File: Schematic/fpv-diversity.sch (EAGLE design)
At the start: 62 parts, among them U1 LM1881M/NOPB, U2 LM1881M/NOPB, U3 LM1881M/NOPB, U4 MAX4545CAP+, U5 LT6206CMS8PBF, U6 LM1117IMP-5.0-NOPB

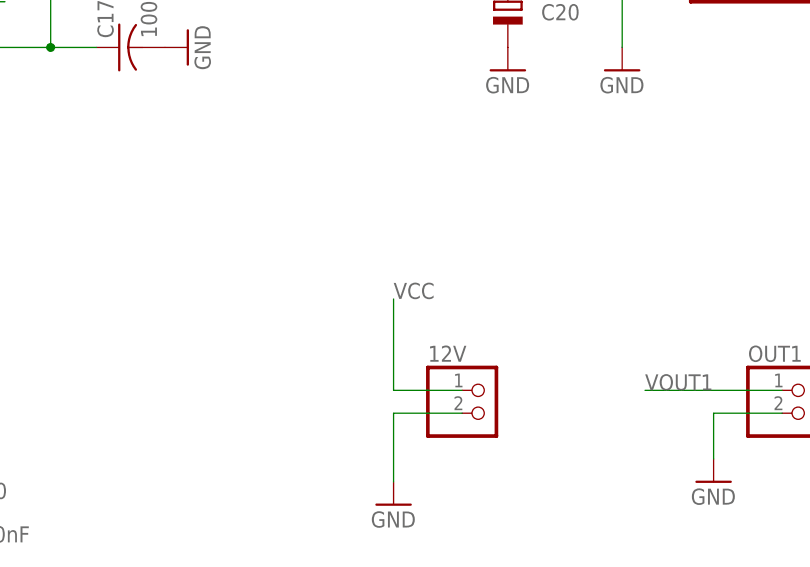
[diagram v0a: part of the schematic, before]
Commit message: Updates
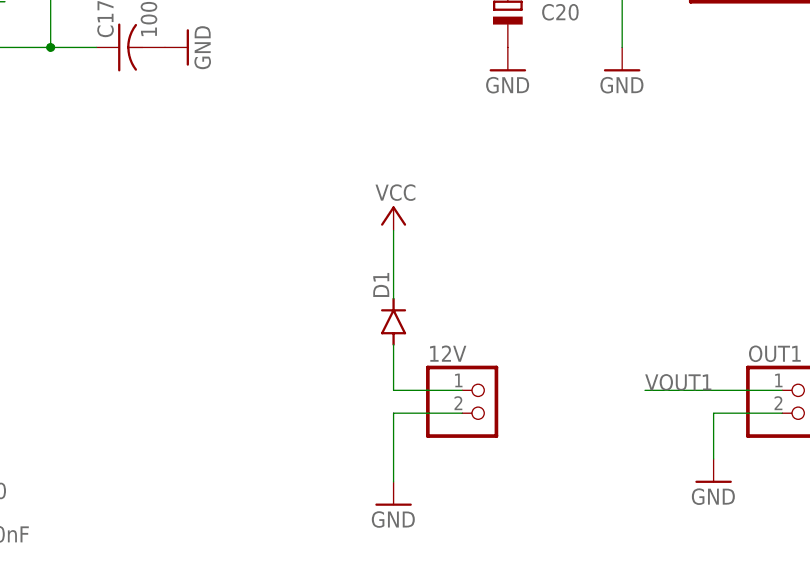
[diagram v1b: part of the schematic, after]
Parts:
- added D1: (no value), diode:DIODE-DO-214AC
- C19, C20: device rcl:CPOL-EUUD-4X5,8 -> rcl:CPOL-EUD/7343-31W
- R1, R10, R11, R12, R14, R15, R17, R18, R3, R7, R8: device rcl:R-US_R1206 -> rcl:R-US_R0805
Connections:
- new net N$6: 12V.1, D1.A
- net VCC: now also D1.C; no longer 12V.1

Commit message: more updates
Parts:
- R13, R2, R9: device rcl:R-US_R1206 -> rcl:R-US_R0805
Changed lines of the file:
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@@
 <part name="C3" library="rcl" library_urn="urn:adsk.eagle:library:334" deviceset="C-US" device="C0805" package3d_urn="urn:adsk.eagle:package:23617/2" value="100nF"/>
 <part name="GND3" library="supply1" library_urn="urn:adsk.eagle:library:371" deviceset="GND" device=""/>
-<part name="R2" library="rcl" library_urn="urn:adsk.eagle:library:334" deviceset="R-US_" device="R1206" package3d_urn="urn:adsk.eagle:package:23540/2" value="75"/>
+<part name="R2" library="rcl" library_urn="urn:adsk.eagle:library:334" deviceset="R-US_" device="R0805" package3d_urn="urn:adsk.eagle:package:23553/2" value="75"/>
 <part name="GND4" library="supply1" library_urn="urn:adsk.eagle:library:371" deviceset="GND" device=""/>
 <part name="U2" library="LM1881M_NOPB" deviceset="LM1881M/NOPB" device="" package3d_urn="urn:adsk.eagle:package:18494142/1"/>
@@
 <part name="C7" library="rcl" library_urn="urn:adsk.eagle:library:334" deviceset="C-US" device="C0805" package3d_urn="urn:adsk.eagle:package:23617/2" value="100nF"/>
 <part name="GND8" library="supply1" library_urn="urn:adsk.eagle:library:371" deviceset="GND" device=""/>
-<part name="R9" library="rcl" library_urn="urn:adsk.eagle:library:334" deviceset="R-US_" device="R1206" package3d_urn="urn:adsk.eagle:package:23540/2" value="75"/>
+<part name="R9" library="rcl" library_urn="urn:adsk.eagle:library:334" deviceset="R-US_" device="R0805" package3d_urn="urn:adsk.eagle:package:23553/2" value="75"/>
 <part name="GND9" library="supply1" library_urn="urn:adsk.eagle:library:371" deviceset="GND" device=""/>
 <part name="U3" library="LM1881M_NOPB" deviceset="LM1881M/NOPB" device="" package3d_urn="urn:adsk.eagle:package:18494142/1"/>
@@
 <part name="C13" library="rcl" library_urn="urn:adsk.eagle:library:334" deviceset="C-US" device="C0805" package3d_urn="urn:adsk.eagle:package:23617/2" value="100nF"/>
 <part name="GND20" library="supply1" library_urn="urn:adsk.eagle:library:371" deviceset="GND" device=""/>
-<part name="R13" library="rcl" library_urn="urn:adsk.eagle:library:334" deviceset="R-US_" device="R1206" package3d_urn="urn:adsk.eagle:package:23540/2" value="75"/>
+<part name="R13" library="rcl" library_urn="urn:adsk.eagle:library:334" deviceset="R-US_" device="R0805" package3d_urn="urn:adsk.eagle:package:23553/2" value="75"/>
 <part name="GND21" library="supply1" library_urn="urn:adsk.eagle:library:371" deviceset="GND" device=""/>
 <part name="U1" library="LM1881M_NOPB" deviceset="LM1881M/NOPB" device="" package3d_urn="urn:adsk.eagle:package:18494142/1"/>

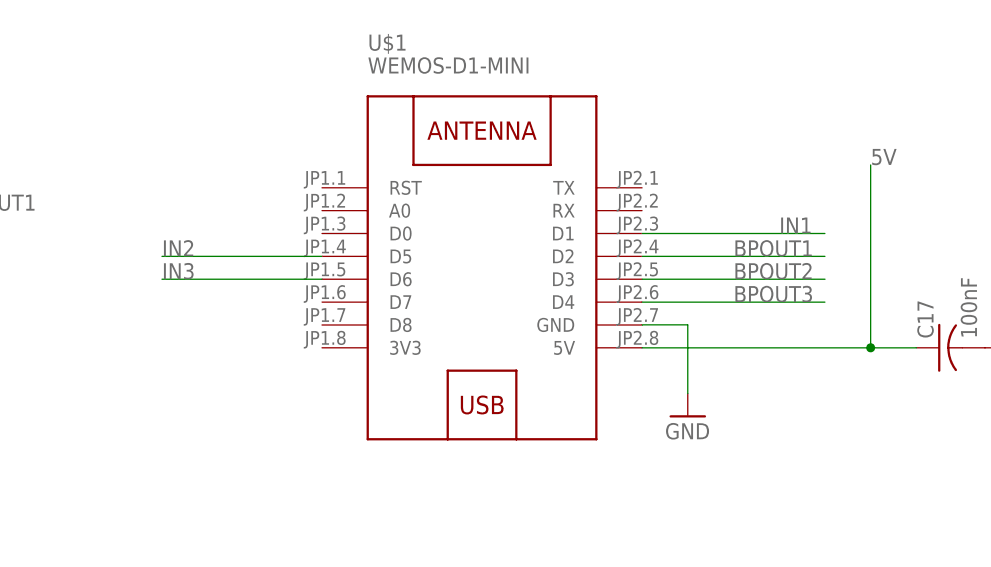
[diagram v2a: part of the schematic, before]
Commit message: Latest
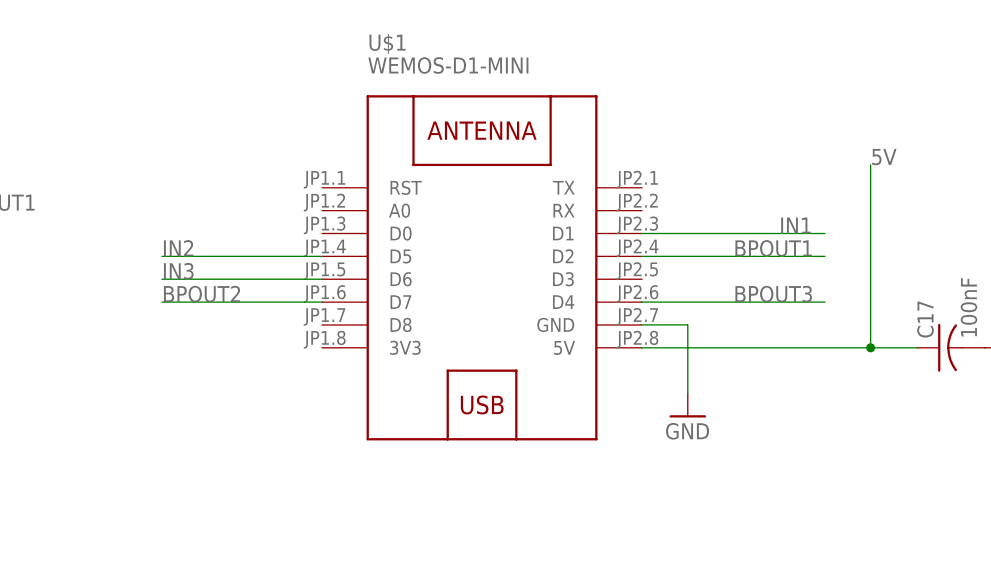
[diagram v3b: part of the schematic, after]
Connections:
- net BPOUT2: now also U$1.D7; no longer U$1.D3
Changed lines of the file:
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@@
 <grid distance="0.1" unitdist="inch" unit="inch" style="lines" multiple="1" display="no" altdistance="0.01" altunitdist="inch" altunit="inch"/>
 <layers>
-<layer number="1" name="Top" color="4" fill="1" visible="yes" active="no"/>
-<layer number="2" name="Route2" color="16" fill="1" visible="yes" active="no"/>
-<layer number="3" name="Route3" color="17" fill="1" visible="yes" active="no"/>
-<layer number="4" name="Route4" color="18" fill="1" visible="yes" active="no"/>
-<layer number="5" name="Route5" color="19" fill="1" visible="yes" active="no"/>
-<layer number="6" name="Route6" color="25" fill="1" visible="yes" active="no"/>
-<layer number="7" name="Route7" color="26" fill="1" visible="yes" active="no"/>
-<layer number="8" name="Route8" color="27" fill="1" visible="yes" active="no"/>
-<layer number="9" name="Route9" color="28" fill="1" visible="yes" active="no"/>
-<layer number="10" name="Route10" color="29" fill="1" visible="yes" active="no"/>
-<layer number="11" name="Route11" color="30" fill="1" visible="yes" active="no"/>
-<layer number="12" name="Route12" color="20" fill="1" visible="yes" active="no"/>
-<layer number="13" name="Route13" color="21" fill="1" visible="yes" active="no"/>
-<layer number="14" name="Route14" color="22" fill="1" visible="yes" active="no"/>
-<layer number="15" name="Route15" color="23" fill="1" visible="yes" active="no"/>
-<layer number="16" name="Bottom" color="1" fill="1" visible="yes" active="no"/>
-<layer number="17" name="Pads" color="2" fill="1" visible="yes" active="no"/>
-<layer number="18" name="Vias" color="2" fill="1" visible="yes" active="no"/>
-<layer number="19" name="Unrouted" color="6" fill="1" visible="yes" active="no"/>
-<layer number="20" name="Dimension" color="24" fill="1" visible="yes" active="no"/>
-<layer number="21" name="tPlace" color="7" fill="1" visible="yes" active="no"/>
-<layer number="22" name="bPlace" color="7" fill="1" visible="yes" active="no"/>
-<layer number="23" name="tOrigins" color="15" fill="1" visible="yes" active="no"/>
-<layer number="24" name="bOrigins" color="15" fill="1" visible="yes" active="no"/>
-<layer number="25" name="tNames" color="7" fill="1" visible="yes" active="no"/>
-<layer number="26" name="bNames" color="7" fill="1" visible="yes" active="no"/>
-<layer number="27" name="tValues" color="7" fill="1" visible="yes" active="no"/>
-<layer number="28" name="bValues" color="7" fill="1" visible="yes" active="no"/>
+<layer number="1" name="Top" color="4" fill="1" visible="no" active="no"/>
+<layer number="2" name="Route2" color="16" fill="1" visible="no" active="no"/>
+<layer number="3" name="Route3" color="17" fill="1" visible="no" active="no"/>
+<layer number="4" name="Route4" color="18" fill="1" visible="no" active="no"/>
+<layer number="5" name="Route5" color="19" fill="1" visible="no" active="no"/>
+<layer number="6" name="Route6" color="25" fill="1" visible="no" active="no"/>
+<layer number="7" name="Route7" color="26" fill="1" visible="no" active="no"/>
+<layer number="8" name="Route8" color="27" fill="1" visible="no" active="no"/>
+<layer number="9" name="Route9" color="28" fill="1" visible="no" active="no"/>
+<layer number="10" name="Route10" color="29" fill="1" visible="no" active="no"/>
+<layer number="11" name="Route11" color="30" fill="1" visible="no" active="no"/>
+<layer number="12" name="Route12" color="20" fill="1" visible="no" active="no"/>
+<layer number="13" name="Route13" color="21" fill="1" visible="no" active="no"/>
+<layer number="14" name="Route14" color="22" fill="1" visible="no" active="no"/>
+<layer number="15" name="Route15" color="23" fill="1" visible="no" active="no"/>
+<layer number="16" name="Bottom" color="1" fill="1" visible="no" active="no"/>
+<layer number="17" name="Pads" color="2" fill="1" visible="no" active="no"/>
+<layer number="18" name="Vias" color="2" fill="1" visible="no" active="no"/>
+<layer number="19" name="Unrouted" color="6" fill="1" visible="no" active="no"/>
+<layer number="20" name="Dimension" color="24" fill="1" visible="no" active="no"/>
+<layer number="21" name="tPlace" color="7" fill="1" visible="no" active="no"/>
+<layer number="22" name="bPlace" color="7" fill="1" visible="no" active="no"/>
+<layer number="23" name="tOrigins" color="15" fill="1" visible="no" active="no"/>
+<layer number="24" name="bOrigins" color="15" fill="1" visible="no" active="no"/>
+<layer number="25" name="tNames" color="7" fill="1" visible="no" active="no"/>
+<layer number="26" name="bNames" color="7" fill="1" visible="no" active="no"/>
+<layer number="27" name="tValues" color="7" fill="1" visible="no" active="no"/>
+<layer number="28" name="bValues" color="7" fill="1" visible="no" active="no"/>
 <layer number="29" name="tStop" color="7" fill="3" visible="no" active="no"/>
 <layer number="30" name="bStop" color="7" fill="6" visible="no" active="no"/>
@@
 <layer number="35" name="tGlue" color="7" fill="4" visible="no" active="no"/>
 <layer number="36" name="bGlue" color="7" fill="5" visible="no" active="no"/>
-<layer number="37" name="tTest" color="7" fill="1" visible="yes" active="no"/>
-<layer number="38" name="bTest" color="7" fill="1" visible="yes" active="no"/>
+<layer number="37" name="tTest" color="7" fill="1" visible="no" active="no"/>
+<layer number="38" name="bTest" color="7" fill="1" visible="no" active="no"/>
 <layer number="39" name="tKeepout" color="4" fill="11" visible="no" active="no"/>
 <layer number="40" name="bKeepout" color="1" fill="11" visible="no" active="no"/>
@@
 <layer number="44" name="Drills" color="7" fill="1" visible="no" active="no"/>
 <layer number="45" name="Holes" color="7" fill="1" visible="no" active="no"/>
-<layer number="46" name="Milling" color="3" fill="1" visible="yes" active="no"/>
-<layer number="47" name="Measures" color="7" fill="1" visible="yes" active="no"/>
-<layer number="48" name="Document" color="7" fill="1" visible="yes" active="no"/>
-<layer number="49" name="Reference" color="7" fill="1" visible="yes" active="no"/>
-<layer number="51" name="tDocu" color="7" fill="1" visible="yes" active="no"/>
-<layer number="52" name="bDocu" color="7" fill="1" visible="yes" active="no"/>
+<layer number="46" name="Milling" color="3" fill="1" visible="no" active="no"/>
+<layer number="47" name="Measures" color="7" fill="1" visible="no" active="no"/>
+<layer number="48" name="Document" color="7" fill="1" visible="no" active="no"/>
+<layer number="49" name="Reference" color="7" fill="1" visible="no" active="no"/>
+<layer number="51" name="tDocu" color="7" fill="1" visible="no" active="no"/>
+<layer number="52" name="bDocu" color="7" fill="1" visible="no" active="no"/>
 <layer number="88" name="SimResults" color="9" fill="1" visible="yes" active="yes"/>
 <layer number="89" name="SimProbes" color="9" fill="1" visible="yes" active="yes"/>
@@
 <part name="GND11" library="supply1" library_urn="urn:adsk.eagle:library:371" deviceset="GND" device=""/>
 <part name="U4" library="MAX4545CAP_" deviceset="MAX4545CAP+" device=""/>
-<part name="U$1" library="diy-modules" deviceset="WEMOS-D1-MINI" device=""/>
+<part name="U$1" library="diy-modules" deviceset="WEMOS-D1-MINI" device="" package3d_urn="urn:adsk.eagle:package:29066244/4"/>
 <part name="GND15" library="supply1" library_urn="urn:adsk.eagle:library:371" deviceset="GND" device=""/>
 <part name="OUT1" library="pinhead" library_urn="urn:adsk.eagle:library:325" deviceset="PINHD-1X2" device="" package3d_urn="urn:adsk.eagle:package:22435/2"/>
@@
 <part name="C17" library="rcl" library_urn="urn:adsk.eagle:library:334" deviceset="C-US" device="C0805" package3d_urn="urn:adsk.eagle:package:23617/2" value="100nF"/>
 <part name="GND25" library="supply1" library_urn="urn:adsk.eagle:library:371" deviceset="GND" device=""/>
-<part name="U6" library="LM1117IMP-5.0-NOPB" deviceset="LM1117IMP-5.0-NOPB" device=""/>
+<part name="U6" library="LM1117IMP-5.0-NOPB" deviceset="LM1117IMP-5.0-NOPB" device="" package3d_urn="urn:adsk.eagle:package:29066744/2"/>
 <part name="GND26" library="supply1" library_urn="urn:adsk.eagle:library:371" deviceset="GND" device=""/>
 <part name="C19" library="rcl" library_urn="urn:adsk.eagle:library:334" deviceset="CPOL-EU" device="D/7343-31W" package3d_urn="urn:adsk.eagle:package:23414/2" value="10uF"/>
@@
 <net name="BPOUT2" class="0">
 <segment>
-<pinref part="U$1" gate="G$1" pin="D3"/>
-<wire x1="208.28" y1="271.78" x2="228.6" y2="271.78" width="0.1524" layer="91"/>
-<label x="218.44" y="271.78" size="1.778" layer="95"/>
-</segment>
-<segment>
 <wire x1="106.68" y1="193.04" x2="116.84" y2="193.04" width="0.1524" layer="91"/>
 <pinref part="C1" gate="G$1" pin="1"/>
@@
 <pinref part="U2" gate="G$1" pin="BPOUT"/>
 </segment>
+<segment>
+<pinref part="U$1" gate="G$1" pin="D7"/>
+<wire x1="172.72" y1="269.24" x2="154.94" y2="269.24" width="0.1524" layer="91"/>
+<label x="154.94" y="269.24" size="1.778" layer="95"/>
+</segment>
 </net>
